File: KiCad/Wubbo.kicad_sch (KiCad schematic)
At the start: 46 parts, among them J2 SWD, J3 USB, J4 JST-BATT, J5 USB, Q1 AO3407, Q2 AO3407, SW1 Choc, SW10 Choc, SW11 Choc, SW12 Choc, SW13 Choc, SW14 Choc, SW15 Choc, SW16 Choc, SW17 Choc, SW2 Choc, SW3 Choc, SW4 Choc, SW5 Choc, SW6 Choc, SW7 Choc, SW8 Choc, SW9 Choc, U1 nRF52840_holyiot_18010, U2 XC6206P LDO, U3 LTC4054ES5-4.2

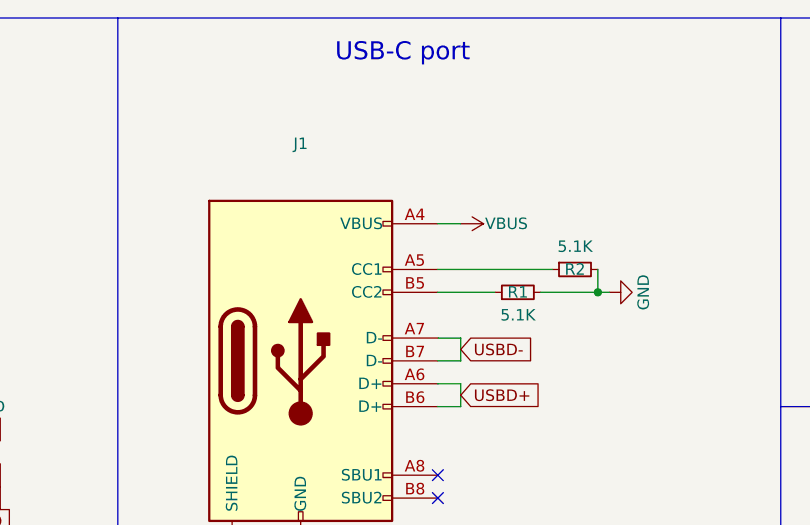
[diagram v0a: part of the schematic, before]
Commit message: wip
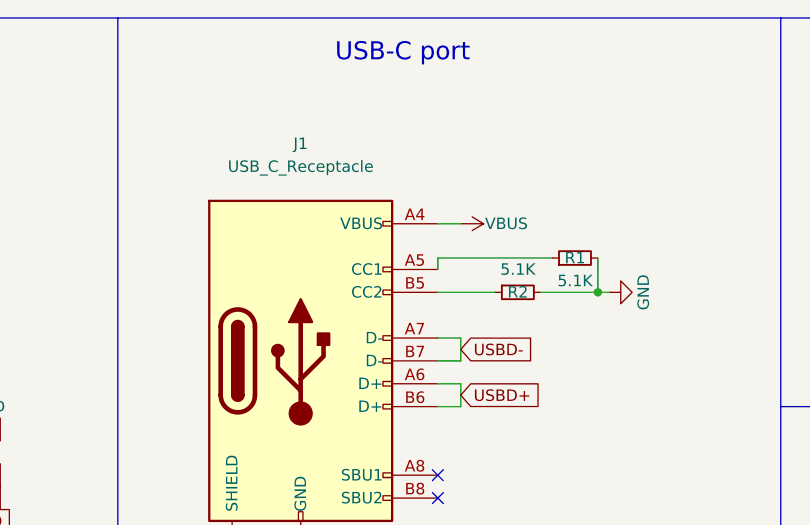
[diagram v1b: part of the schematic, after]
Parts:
- C3: footprint Capacitor_SMD:C_1206_3216Metric -> Capacitor_SMD:C_0805_2012Metric
- D1: footprint LED_SMD:LED_0603_1608Metric -> kiboard_cache:LED_0603_1608Metric_shinethrough
- J1: value (none) -> USB_C_Receptacle; footprint (none) -> USB-C-12-Pin-MidMount
- J2, J3: footprint Connector_PinSocket_1.00mm:PinSocket_1x04_P1.00mm_Vertical -> Connector_PinSocket_2.00mm:PinSocket_1x04_P2.00mm_Vertical
- R10: footprint Resistor_SMD:R_0805_2012Metric -> Resistor_SMD:R_0603_1608Metric
- R_TACT1: footprint Button_Switch_SMD:SW_SPST_EVQP7C -> kiboard_cache:3-4-2_micro_tact_switch
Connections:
- net at R2.1: now also J1.B5 (CC2); no longer J1.A5 (CC1)
- net at R1.1: now also J1.A5 (CC1); no longer J1.B5 (CC2)
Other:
- moved on the sheet: R1, R2
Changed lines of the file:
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@@
+    (stroke (width 0) (type default) (color 0 0 0 0))
+  )
+  (wire (pts (xy 127 39.37) (xy 127 40.64))
     (stroke (width 0) (type default) (color 0 0 0 0))
   )
@@
     (stroke (width 0) (type default) (color 0 0 0 0))
   )
+  (wire (pts (xy 139.7 39.37) (xy 127 39.37))
+    (stroke (width 0) (type default) (color 0 0 0 0))
+  )
   (wire (pts (xy 25.4 140.97) (xy 20.32 140.97))
     (stroke (width 0) (type default) (color 0 0 0 0))
@@
     (stroke (width 0) (type default) (color 0 0 0 0))
   )
+  (wire (pts (xy 127 43.18) (xy 133.35 43.18))
+    (stroke (width 0) (type default) (color 0 0 0 0))
+  )
   (wire (pts (xy 226.06 153.67) (xy 226.06 165.1))
     (stroke (width 0) (type default) (color 0 0 0 0))
@@
     (stroke (width 0) (type default) (color 0 0 0 0))
   )
-  (wire (pts (xy 138.43 43.18) (xy 144.78 43.18))
+  (wire (pts (xy 144.78 39.37) (xy 144.78 43.18))
     (stroke (width 0) (type default) (color 0 0 0 0))
   )
@@
     (stroke (width 0) (type default) (color 0 0 0 0))
   )
-  (wire (pts (xy 127 40.64) (xy 139.7 40.64))
-    (stroke (width 0) (type default) (color 0 0 0 0))
-  )
-  (wire (pts (xy 127 43.18) (xy 133.35 43.18))
-    (stroke (width 0) (type default) (color 0 0 0 0))
-  )
   (wire (pts (xy 259.08 176.53) (xy 259.08 180.34))
     (stroke (width 0) (type default) (color 0 0 0 0))
@@
     (stroke (width 0) (type default) (color 0 0 0 0))
   )
-  (wire (pts (xy 144.78 43.18) (xy 144.78 40.64))
+  (wire (pts (xy 144.78 43.18) (xy 138.43 43.18))
     (stroke (width 0) (type default) (color 0 0 0 0))
   )
@@
       (effects (font (size 1.27 1.27)) (justify right))
     )
-    (property "Footprint" "Button_Switch_SMD:SW_SPST_EVQP7C" (id 2) (at 254 83.82 0)
+    (property "Footprint" "kiboard_cache:3-4-2_micro_tact_switch" (id 2) (at 254 83.82 0)
       (effects (font (size 1.27 1.27)) hide)
     )
@@
     (pin "3")
   )
-  (symbol (lib_id "Device:R_Small") (at 142.24 40.64 90) (mirror x) (unit 1)
-    (in_bom yes) (on_board yes)
-    (property "Reference" "R2" (id 0) (at 142.24 40.64 90))
-    (property "Value" "5.1K" (id 1) (at 142.24 38.1 90))
-    (property "Footprint" "Resistor_SMD:R_0603_1608Metric" (id 2) (at 142.24 40.64 0)
-      (effects (font (size 1.27 1.27)) hide)
-    )
-    (property "Datasheet" "~" (id 3) (at 142.24 40.64 0)
+  (symbol (lib_id "Device:R_Small") (at 135.89 43.18 90) (mirror x) (unit 1)
+    (in_bom yes) (on_board yes)
+    (property "Reference" "R2" (id 0) (at 135.89 43.18 90))
+    (property "Value" "5.1K" (id 1) (at 135.89 40.64 90))
+    (property "Footprint" "Resistor_SMD:R_0603_1608Metric" (id 2) (at 135.89 43.18 0)
+      (effects (font (size 1.27 1.27)) hide)
+    )
+    (property "Datasheet" "~" (id 3) (at 135.89 43.18 0)
       (effects (font (size 1.27 1.27)) hide)
     )
@@
     (pin "2")
   )
-  (symbol (lib_id "Device:R_Small") (at 135.89 43.18 90) (unit 1)
-    (in_bom yes) (on_board yes)
-    (property "Reference" "R1" (id 0) (at 135.89 43.18 90))
-    (property "Value" "5.1K" (id 1) (at 135.89 45.72 90))
-    (property "Footprint" "Resistor_SMD:R_0603_1608Metric" (id 2) (at 135.89 43.18 0)
-      (effects (font (size 1.27 1.27)) hide)
-    )
-    (property "Datasheet" "~" (id 3) (at 135.89 43.18 0)
+  (symbol (lib_id "Device:R_Small") (at 142.24 39.37 90) (unit 1)
+    (in_bom yes) (on_board yes)
+    (property "Reference" "R1" (id 0) (at 142.24 39.37 90))
+    (property "Value" "5.1K" (id 1) (at 142.24 41.91 90))
+    (property "Footprint" "Resistor_SMD:R_0603_1608Metric" (id 2) (at 142.24 39.37 0)
+      (effects (font (size 1.27 1.27)) hide)
+    )
+    (property "Datasheet" "~" (id 3) (at 142.24 39.37 0)
       (effects (font (size 1.27 1.27)) hide)
     )
@@
     (property "Reference" "R10" (id 0) (at 110.49 87.7316 90))
     (property "Value" "1M" (id 1) (at 110.49 90.043 90))
-    (property "Footprint" "Resistor_SMD:R_0805_2012Metric" (id 2) (at 110.49 92.71 0)
+    (property "Footprint" "Resistor_SMD:R_0603_1608Metric" (id 2) (at 110.49 92.71 0)
       (effects (font (size 1.27 1.27)) hide)
     )
@@
     (property "Reference" "D1" (id 0) (at 190.5 95.25 0))
     (property "Value" "Blue LED" (id 1) (at 190.5 92.71 0))
-    (property "Footprint" "LED_SMD:LED_0603_1608Metric" (id 2) (at 190.5 88.9 0)
+    (property "Footprint" "kiboard_cache:LED_0603_1608Metric_shinethrough" (id 2) (at 190.5 88.9 0)
       (effects (font (size 1.27 1.27)) hide)
     )
@@
     (property "Reference" "C3" (id 0) (at 110.49 94.5134 90))
     (property "Value" "4.7n" (id 1) (at 110.49 96.8248 90))
-    (property "Footprint" "Capacitor_SMD:C_1206_3216Metric" (id 2) (at 110.49 100.33 0)
+    (property "Footprint" "Capacitor_SMD:C_0805_2012Metric" (id 2) (at 110.49 100.33 0)
       (effects (font (size 1.27 1.27)) hide)
     )
@@
       (effects (font (size 1.27 1.27)) (justify left))
     )
-    (property "Footprint" "Connector_PinSocket_1.00mm:PinSocket_1x04_P1.00mm_Vertical" (id 2) (at 275.59 109.22 0)
+    (property "Footprint" "Connector_PinSocket_2.00mm:PinSocket_1x04_P2.00mm_Vertical" (id 2) (at 275.59 109.22 0)
       (effects (font (size 1.27 1.27)) hide)
     )
@@
       (effects (font (size 1.27 1.27)) (justify left))
     )
-    (property "Footprint" "Connector_PinSocket_1.00mm:PinSocket_1x04_P1.00mm_Vertical" (id 2) (at 245.11 109.22 0)
+    (property "Footprint" "Connector_PinSocket_2.00mm:PinSocket_1x04_P2.00mm_Vertical" (id 2) (at 245.11 109.22 0)
       (effects (font (size 1.27 1.27)) hide)
     )
@@
     (in_bom yes) (on_board yes)
     (property "Reference" "J1" (id 0) (at 111.76 26.67 0))
-    (property "Value" "" (id 1) (at 111.76 29.21 0))
-    (property "Footprint" "" (id 2) (at 115.57 50.8 0)
+    (property "Value" "USB_C_Receptacle" (id 1) (at 111.76 29.21 0))
+    (property "Footprint" "USB-C-12-Pin-MidMount" (id 2) (at 115.57 50.8 0)
       (effects (font (size 1.27 1.27)) hide)
     )
@@
     )
     (path "/a4ad2a42-7fbf-4229-aa42-a4b8c66f5d7d"
-      (reference "C3") (unit 1) (value "4.7n") (footprint "Capacitor_SMD:C_1206_3216Metric")
+      (reference "C3") (unit 1) (value "4.7n") (footprint "Capacitor_SMD:C_0805_2012Metric")
     )
     (path "/a3a73473-160c-433a-9e43-57c439fa600c"
-      (reference "D1") (unit 1) (value "Blue LED") (footprint "LED_SMD:LED_0603_1608Metric")
+      (reference "D1") (unit 1) (value "Blue LED") (footprint "kiboard_cache:LED_0603_1608Metric_shinethrough")
     )
     (path "/b936b398-3ee7-4074-bb47-f4265b1e3df1"
@@
     )
     (path "/c43e2dd7-a96c-4da8-8a15-5019b7dc39dd"
-      (reference "J2") (unit 1) (value "SWD") (footprint "Connector_PinSocket_1.00mm:PinSocket_1x04_P1.00mm_Vertical")
+      (reference "J2") (unit 1) (value "SWD") (footprint "Connector_PinSocket_2.00mm:PinSocket_1x04_P2.00mm_Vertical")
     )
     (path "/b6756e26-1517-439a-935c-3bc234c0d963"
-      (reference "J3") (unit 1) (value "USB") (footprint "Connector_PinSocket_1.00mm:PinSocket_1x04_P1.00mm_Vertical")
+      (reference "J3") (unit 1) (value "USB") (footprint "Connector_PinSocket_2.00mm:PinSocket_1x04_P2.00mm_Vertical")
     )
     (path "/596ada96-a989-46ff-8abe-ba8f0b70ba7d"
@@
     )
     (path "/94b6b5f0-f01b-4ffa-a5fa-84fa522d0ba9"
-      (reference "R10") (unit 1) (value "1M") (footprint "Resistor_SMD:R_0805_2012Metric")
+      (reference "R10") (unit 1) (value "1M") (footprint "Resistor_SMD:R_0603_1608Metric")
     )
     (path "/245d5d07-bad9-4ecb-9c30-e7954a9c9422"
-      (reference "R_TACT1") (unit 1) (value "SW_Push") (footprint "Button_Switch_SMD:SW_SPST_EVQP7C")
+      (reference "R_TACT1") (unit 1) (value "SW_Push") (footprint "kiboard_cache:3-4-2_micro_tact_switch")
     )
     (path "/ae2bde3b-d71e-46a6-80d9-110327765c83"
